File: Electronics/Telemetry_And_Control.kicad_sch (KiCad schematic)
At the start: 16 parts, among them J1 Micro_SD_Card_Det_Hirose_DM3AT, U5 ESP32-S3-WROOM-1

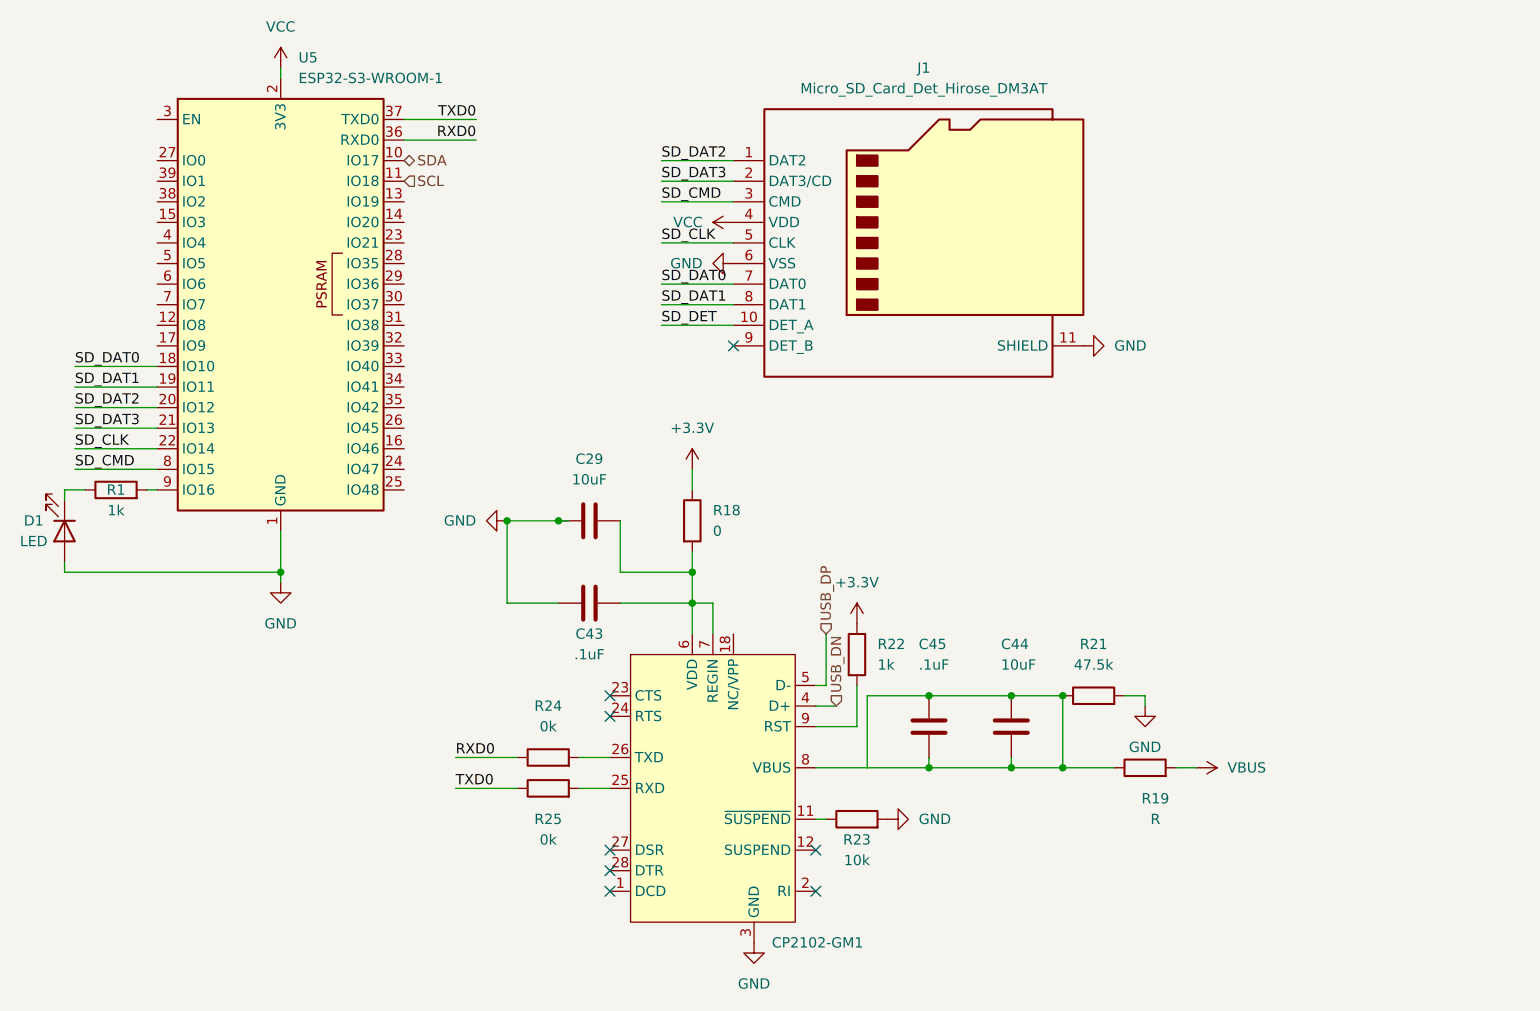
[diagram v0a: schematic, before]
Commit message: mostly done, needs review, needs pins
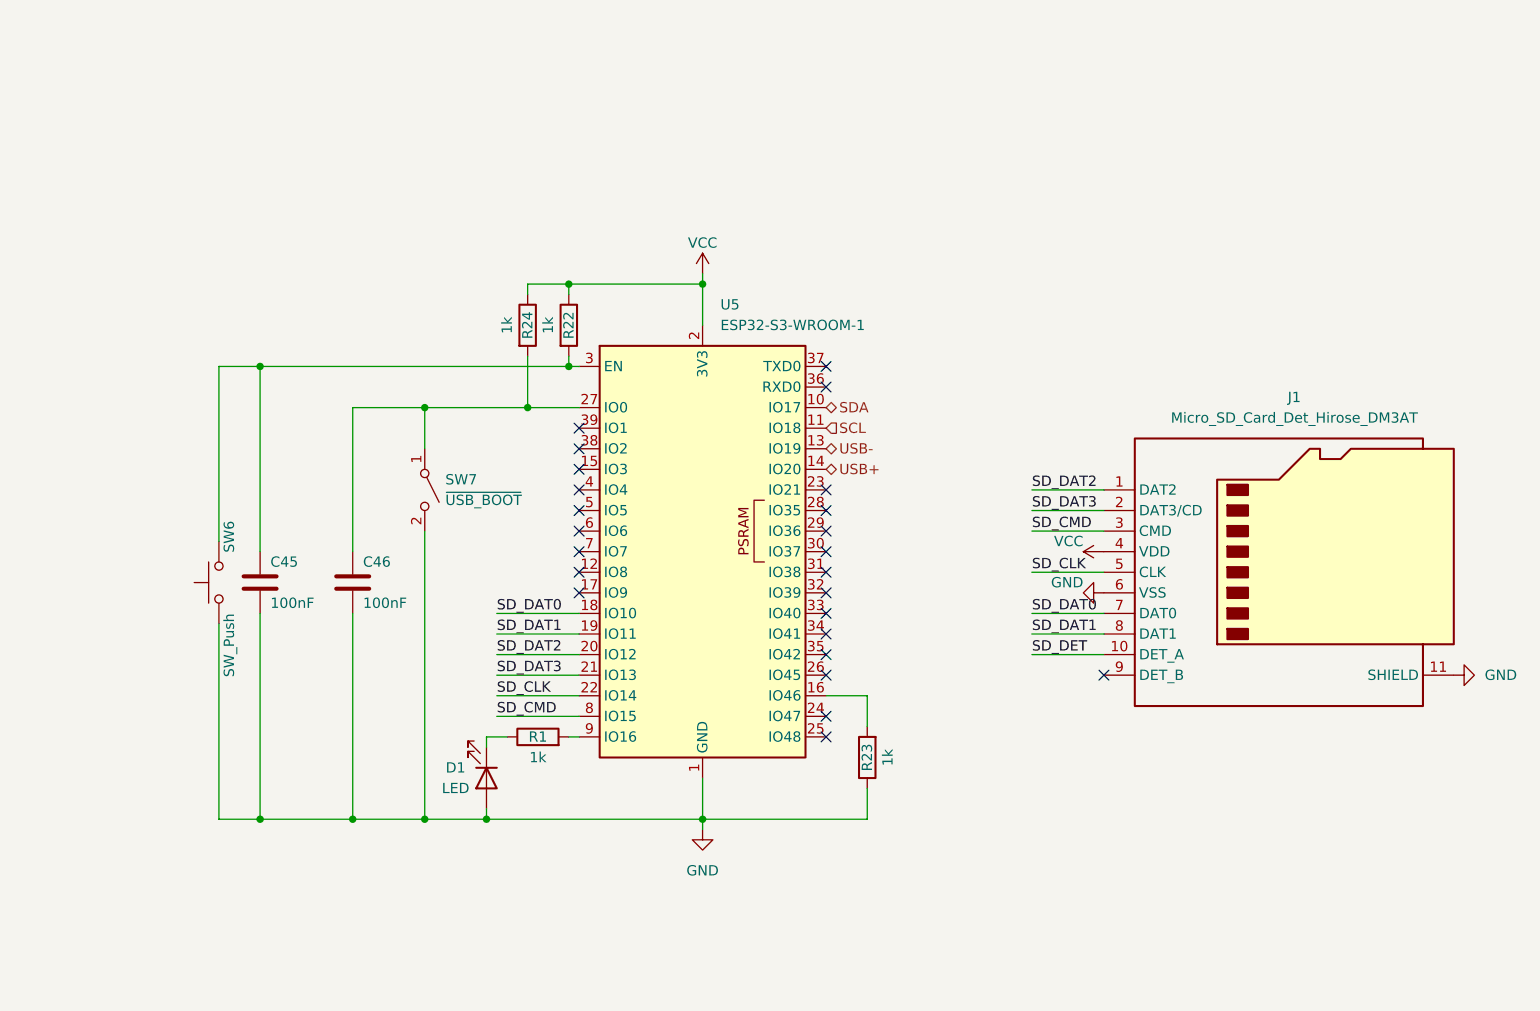
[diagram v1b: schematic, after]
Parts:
- removed C29, C44: 10uF, symbol Device:C
- removed C43: .1uF, symbol Device:C
- removed CP2102-GM1: ~, Package_DFN_QFN:QFN-28-1EP_5x5mm_P0.5mm_EP3.1x3.1mm, symbol CP2102-GM:CP2102-GM
- removed R18: 0, symbol Device:R
- removed R19: R, symbol Device:R
- removed R21: 47.5k, symbol Device:R
- removed R25: 0k, symbol Device:R
- added C46: 100nF, symbol Device:C
- added SW6: SW_Push, symbol Switch:SW_Push
- added SW7: ~{USB_BOOT}, symbol Switch:SW_SPST
- C45: value .1uF -> 100nF
- R22: footprint (none) -> Resistor_SMD:R_0201_0603Metric
- R23: value 10k -> 1k; footprint (none) -> Resistor_SMD:R_0201_0603Metric
- R24: value 0k -> 1k; footprint (none) -> Resistor_SMD:R_0201_0603Metric
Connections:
- net +3.3V is gone; now on net VCC: R22.1
- net GND: now also C45.2, R23.1, C46.2, SW6.1, SW7.2 (B); no longer R23.2
- net VCC: now also R24.1
- net at C45.1: now also R22.2, U5.3 (EN), SW6.2; no longer C45.2
- net at R24.2: now also U5.27 (IO0), C46.1, SW7.1 (A)
- net USB-: now reaches U5.13 (IO19)
- net USB+: now reaches U5.14 (IO20)
- net at U5.16 (IO46): now also R23.2
- net RXD0: no longer names the net of U5.36 (RXD0)
- net RXD0: no longer R24.1
- net TXD0: no longer names the net of U5.37 (TXD0)
- no-connect marks 8 -> 24
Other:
- moved on the sheet: D1, J1, R1, U5
